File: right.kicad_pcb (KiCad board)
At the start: 2 copper layers, 152.4 x 109.7 mm, 67 parts, among them U1 74VHC4051AFT, U2 GS8051-TR, U3 ATMEGA32U4, U4 PJ-327A, Y1 Crystal

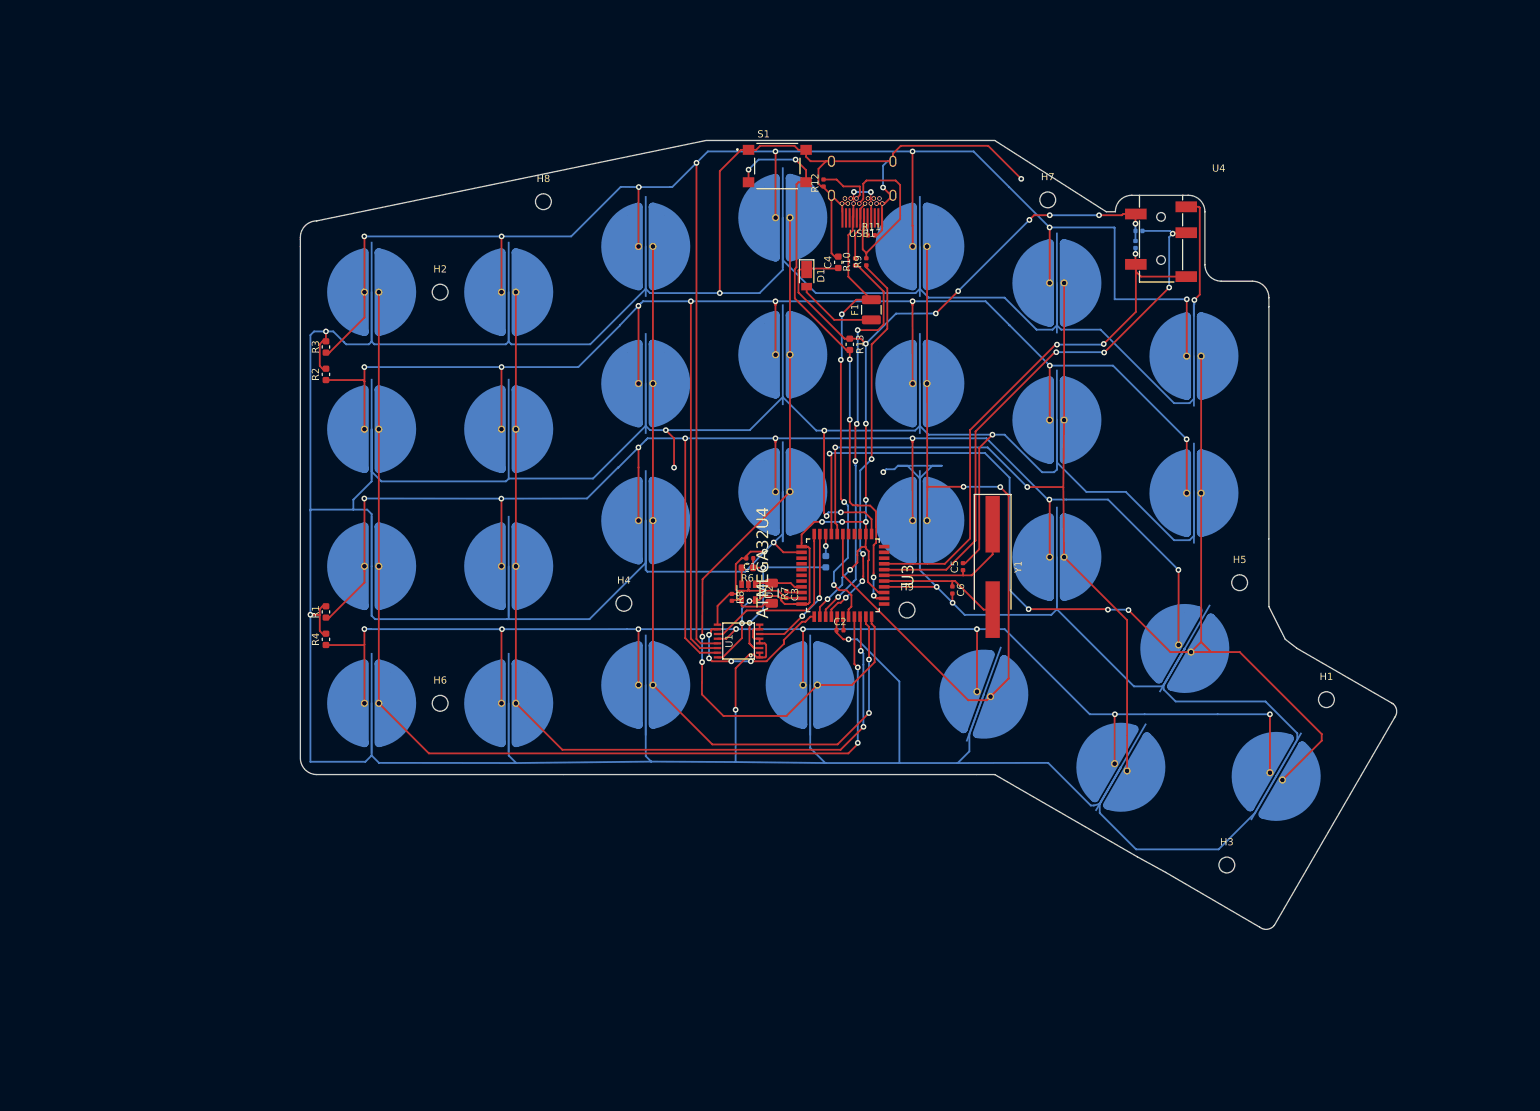
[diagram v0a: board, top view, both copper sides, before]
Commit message: fill
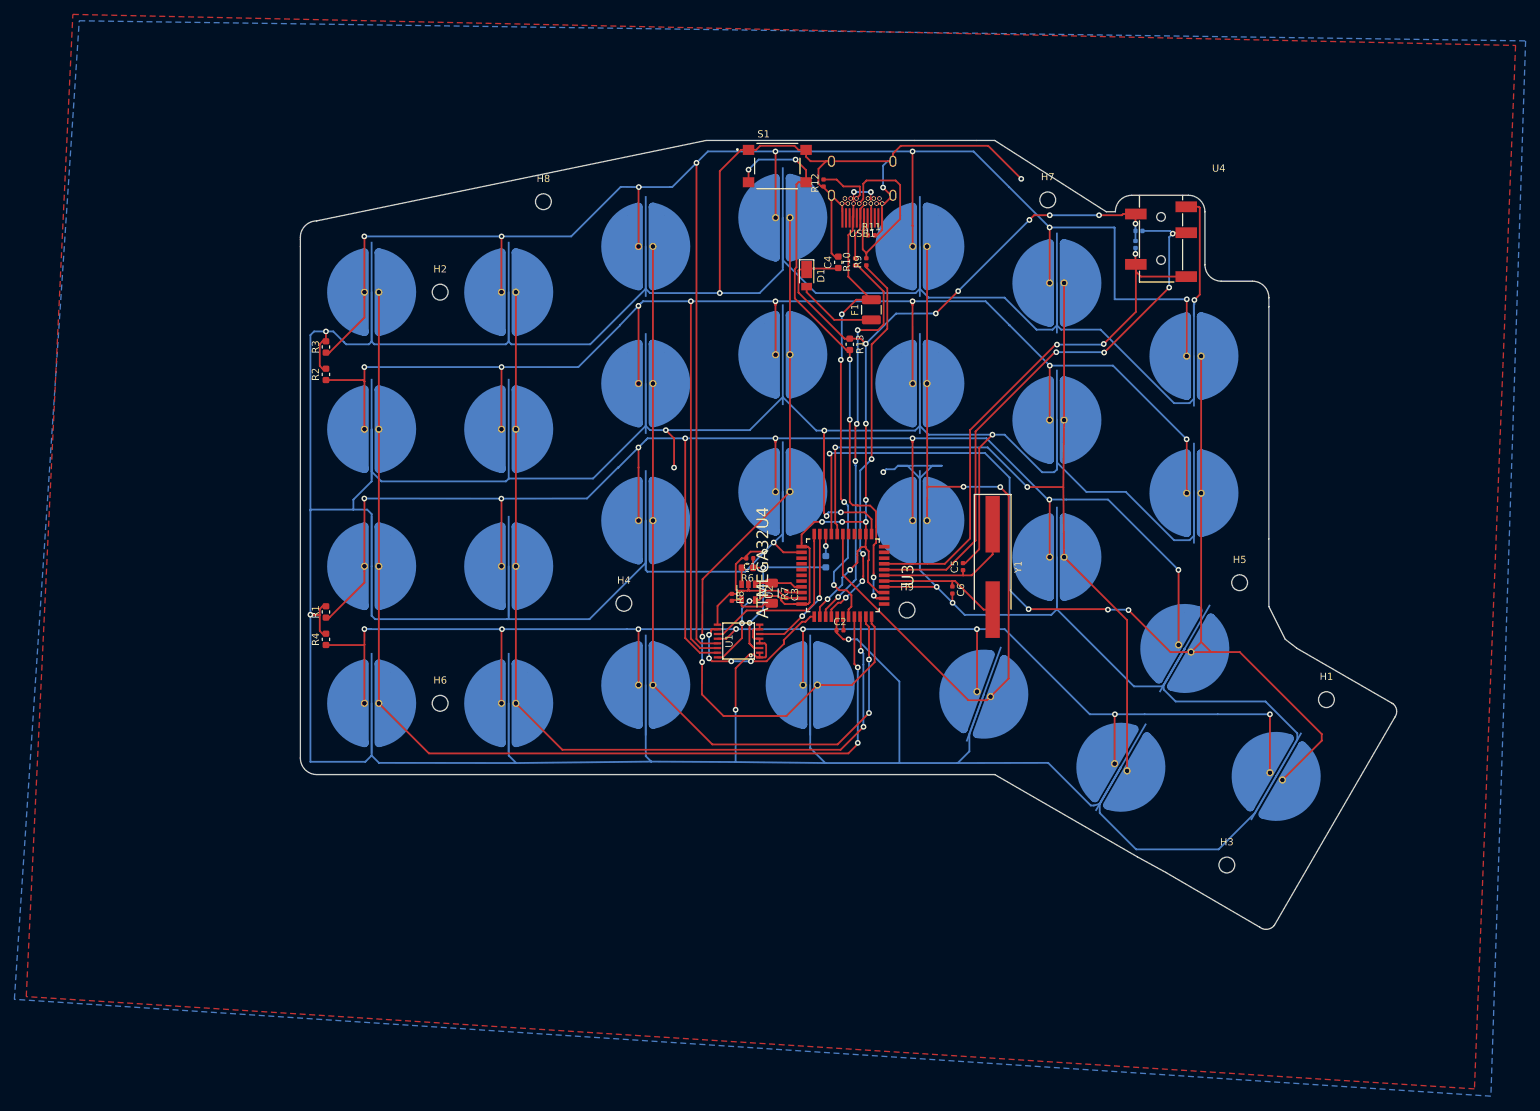
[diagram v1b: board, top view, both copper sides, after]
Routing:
- added copper zone on B.Cu, net GND
- added copper zone on F.Cu, net GND
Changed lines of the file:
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@@
+    )
+  )
+  (zone (net 1) (net_name GND) (layer F.Cu) (hatch edge 0.508)
+    (connect_pads (clearance 0.508))
+    (min_thickness 0.254)
+    (fill yes (arc_segments 32) (thermal_gap 0.508) (thermal_bridge_width 0.508))
+    (polygon
+      (pts
+        (xy 247.142 41.656) (xy 241.427 186.69) (xy 40.132 173.863) (xy 46.609 37.338)
+      )
+    )
+  )
+  (zone (net 1) (net_name GND) (layer B.Cu) (hatch edge 0.508)
+    (connect_pads (clearance 0.508))
+    (min_thickness 0.254)
+    (fill yes (arc_segments 32) (thermal_gap 0.508) (thermal_bridge_width 0.508))
+    (polygon
+      (pts
+        (xy 248.539 41.021) (xy 243.713 187.706) (xy 38.481 174.244) (xy 47.498 38.227)
+      )
     )
   )
